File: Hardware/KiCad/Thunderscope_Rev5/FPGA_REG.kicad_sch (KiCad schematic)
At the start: 48 parts, among them U20 TPS62A02, U21 TPS62A02, U22 TPS7A9101, U23 TPS62A02, U24 TPS22975

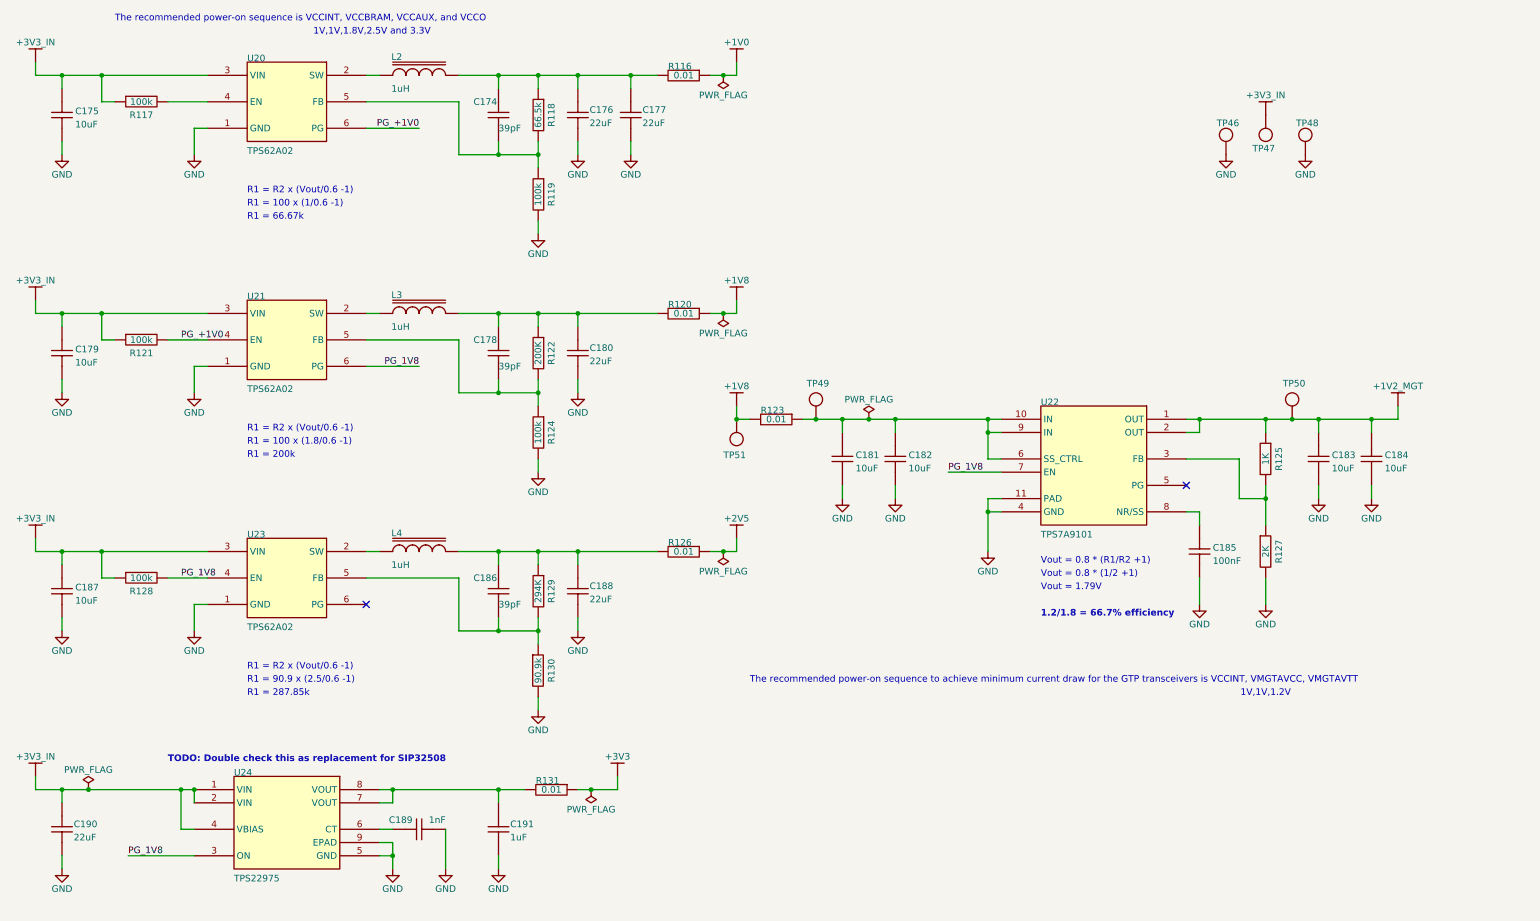
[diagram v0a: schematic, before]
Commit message: Added WIP Mech Model and Interposer
Also reworked rev5 power tree
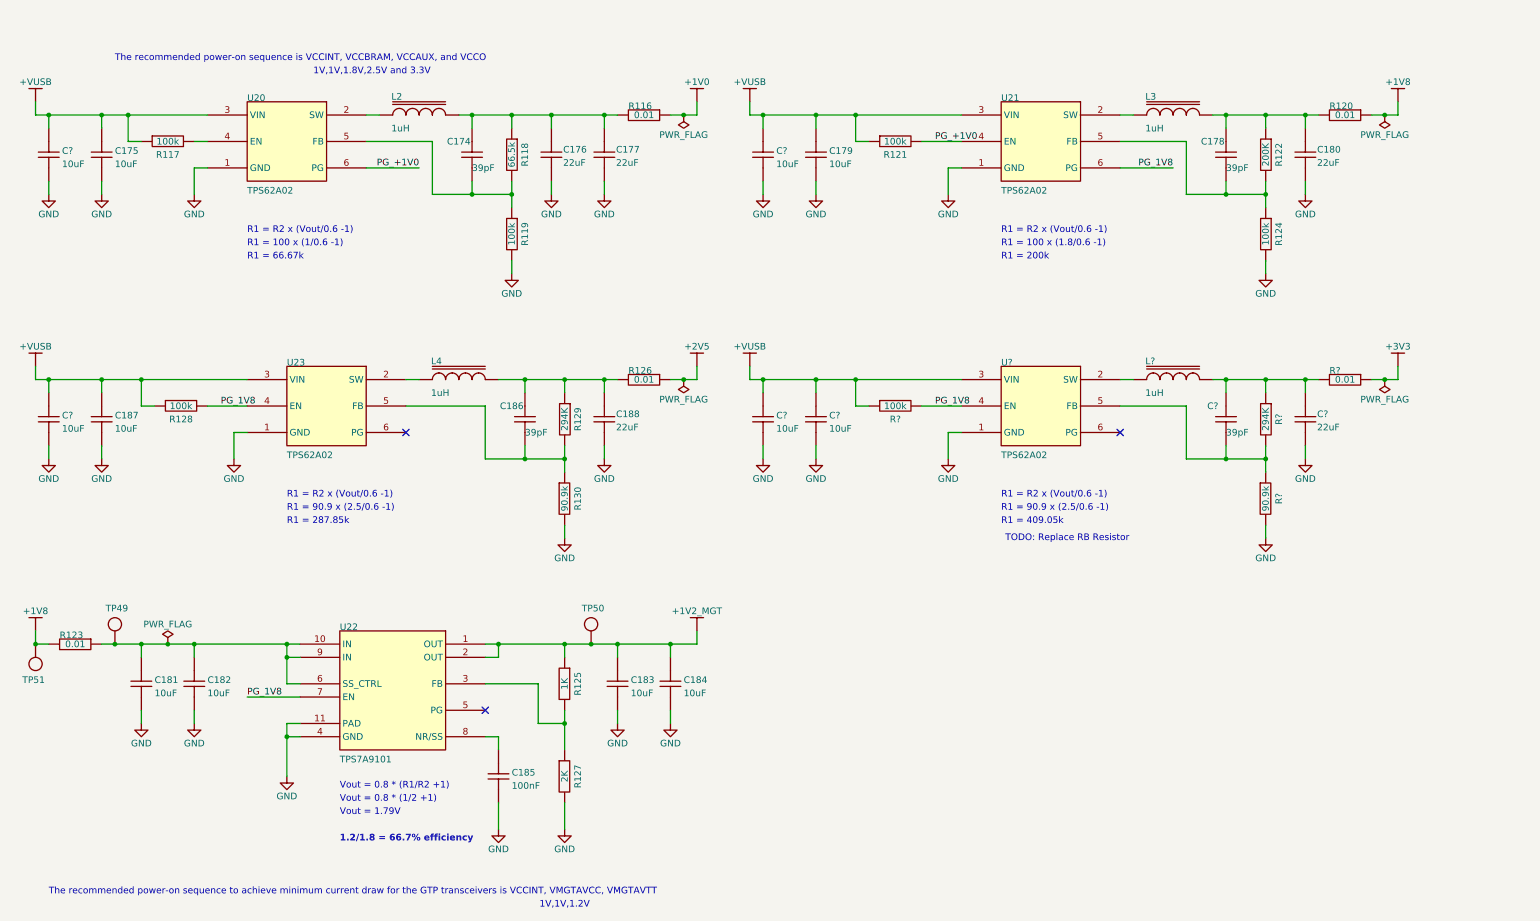
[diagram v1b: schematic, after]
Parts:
- removed C189: ${ALTIUM_VALUE}, GEN_C_0402, symbol Thunderscope_Rev5:CAP 1nF 50V C0G 0402
- removed C190: ${ALTIUM_VALUE}, GEN_C_0805, symbol Thunderscope_Rev5:CAP 22uF 25V X5R 0805
- removed C191: ${ALTIUM_VALUE}, GEN_C_0402, symbol Thunderscope_Rev5:CAP 1uF 25V X5R 0402
- removed R131: ${ALTIUM_VALUE}, GEN_R_0603, symbol Thunderscope_Rev5:RES 0.01 OHM 1% 1/4W 0603
- removed TP46, TP47, TP48: PCB, GEN_TP_PCB, symbol Thunderscope_Rev5:TP PCB 1mm
- removed U24: TPS22975, TI_WSON8_DSG0008A, symbol Thunderscope_Rev5:IC SWITCH LOAD TPS22975
- added C? (x5): ${ALTIUM_VALUE}, GEN_C_0603, symbol Thunderscope_Rev5:CAP 10uF 10V X5R 0603
- added C?: ${ALTIUM_VALUE}, GEN_C_0805, symbol Thunderscope_Rev5:CAP 22uF 25V X5R 0805
- added C?: ${ALTIUM_VALUE}, GEN_C_0402, symbol Thunderscope_Rev5:CAP 39pF 50V C0G 0402
- added L?: ${ALTIUM_VALUE}, GEN_L_1210, symbol Thunderscope_Rev5:IND 1uH 5.5A 32 MOHM 1210
- added R?: ${ALTIUM_VALUE}, GEN_R_0402, symbol Thunderscope_Rev5:RES 90.9K OHM 1% 1/16W 0402
- added R?: ${ALTIUM_VALUE}, GEN_R_0402, symbol Thunderscope_Rev5:RES 100K OHM 1% 1/10W 0402
- added R?: ${ALTIUM_VALUE}, GEN_R_0402, symbol Thunderscope_Rev5:RES 294K OHM 1% 1/16W 0402
- added R?: ${ALTIUM_VALUE}, GEN_R_0603, symbol Thunderscope_Rev5:RES 0.01 OHM 1% 1/4W 0603
- added U?: TPS62A02, TI_SOT563_DRL0006A, symbol Thunderscope_Rev5:IC BUCK TPS62A02
- TP49, TP50, TP51: now left out of the parts list
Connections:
- net +3V3: now also R?.2
- net GND: now also C?.1, C?.1, C?.1, C?.1, C?.1, C?.1, R?.2, U?.1 (GND)
- net PG_1V8: now also R?.1, U?.4 (EN)
- net +3V3_IN renamed +VUSB
- net +VUSB: now also C?.2, C?.2, C?.2, C?.2, C?.2, R?.2, U?.3 (VIN)
- new net: L?.1, U?.2 (SW)
- new net: C?.1, R?.1, R?.1, U?.5 (FB)
- new net: C?.2, C?.2, L?.2, R?.1, R?.2
- no-connect marks 2 -> 3
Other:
- note added: "R1 = 409.05k"
- note added: "TODO: Replace RB Resistor"
- note removed: "TODO: Double check this as replacement for SIP32508"
- moved on the sheet: C174, C175, C176, C177, C178, C179, C180, C181, C182, C183, C184, C185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
